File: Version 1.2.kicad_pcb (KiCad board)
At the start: 4 copper layers, 40 x 40 mm, 33 parts, among them J1 Conn_01x04_Pin, J2 Screw_Terminal_01x02, J3 Conn_01x07_Pin, J4 Conn_Coaxial, U1 BGA2801, U2 BGA420, U3 AS179-92LF, U4 SX1278, U5 74LVC1G19, Y1 ECS-TXO-2520-33-400-AN-TR

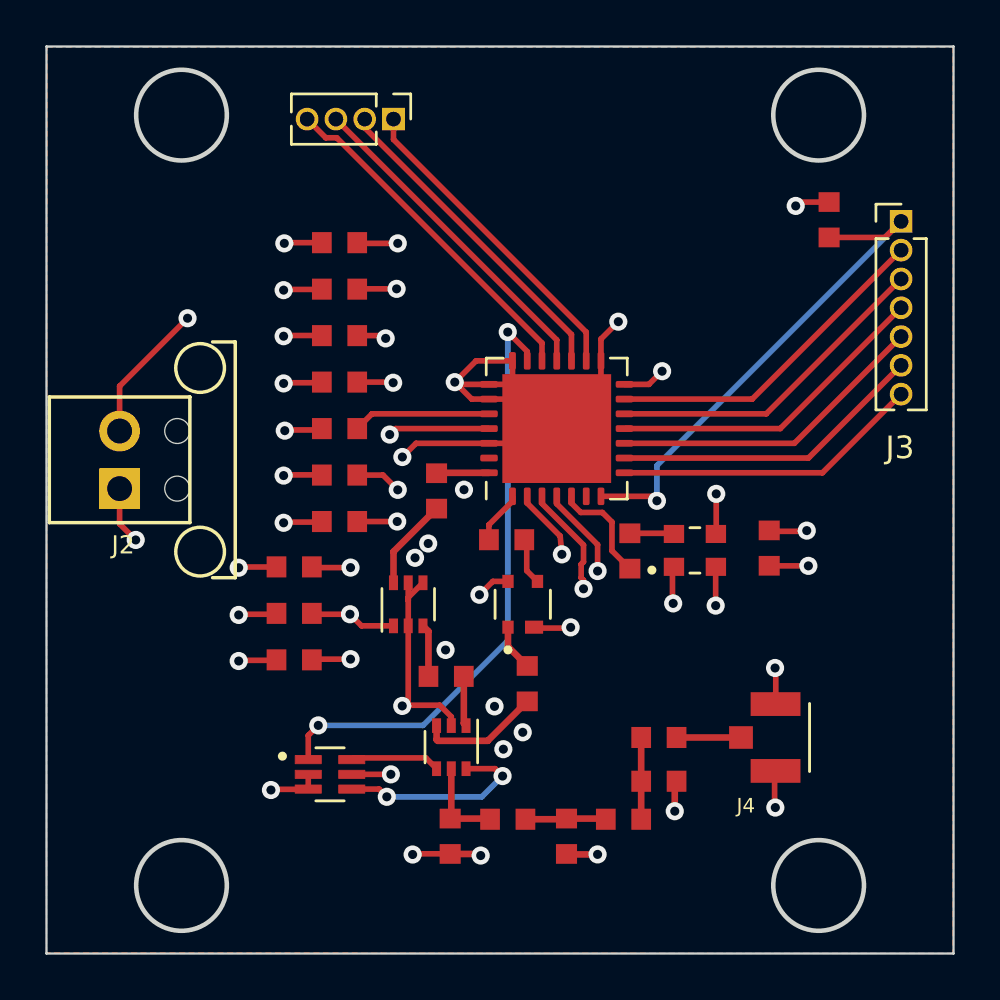
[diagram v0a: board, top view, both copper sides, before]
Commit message: EMI & Compression
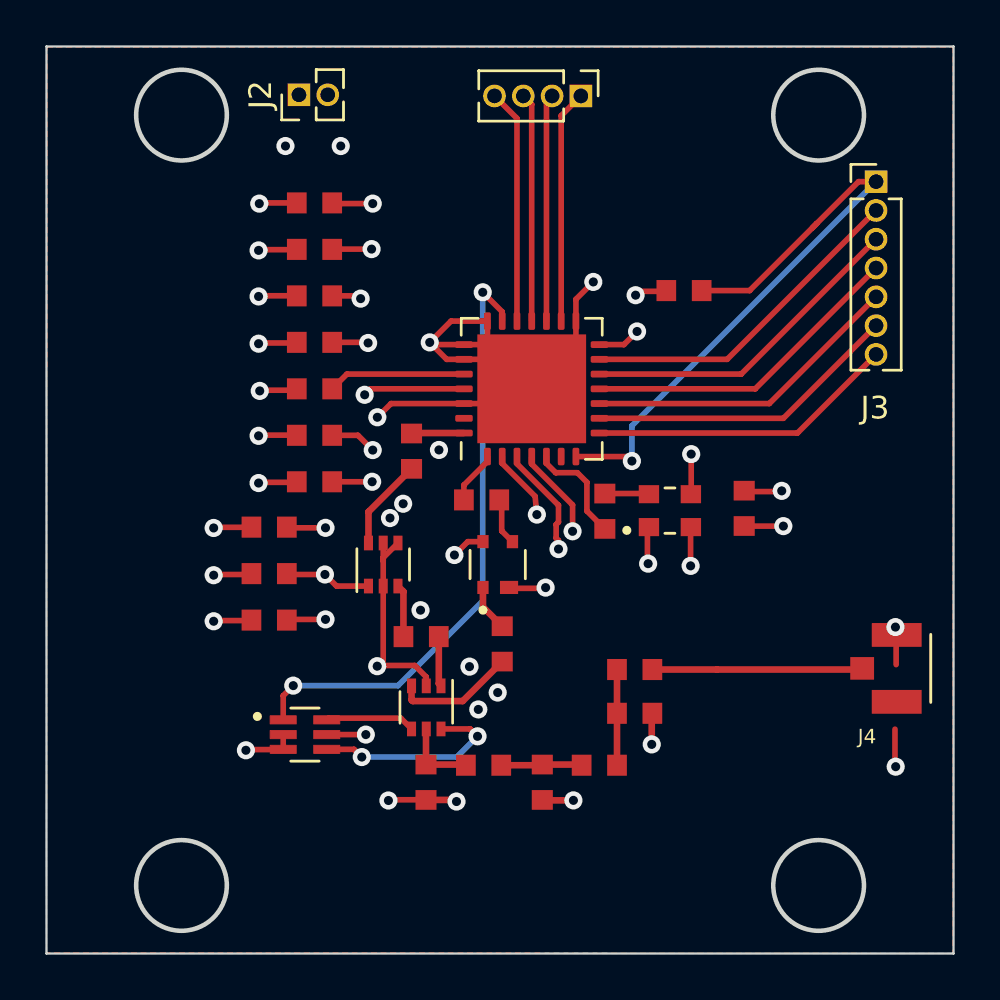
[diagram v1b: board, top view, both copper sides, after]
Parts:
- J2: value Screw_Terminal_01x02 -> Conn_01x02_Pin; footprint Screw Connector 01x02:1725656 -> Connector_PinHeader_1.27mm:PinHeader_1x02_P1.27mm_Vertical
- moved J2 16.3 mm to (127.6, 71.4)
- moved J1 8.33 mm to (140.1, 71.5)
- moved R1 7.12 mm to (144.6, 80.1), turned to 0 degrees
- moved J4 6.15 mm to (154.0, 96.7)
- moved C5 3.18 mm to (142.5, 98.7)
- moved L3 3.18 mm to (142.5, 96.8)
- moved C1 2.61 mm to (133.2, 101.7)
- moved C4 2.61 mm to (138.4, 101.7)
- moved L1 2.61 mm to (135.8, 101.0)
- moved L2 2.61 mm to (140.9, 101.0)
- moved J3 2.07 mm to (153.1, 75.3)
- moved U2 2.07 mm to (136.4, 92.1)
- moved U3 2.07 mm to (133.3, 98.4)
- moved U4 2.07 mm to (137.9, 84.4)
- moved Y1 2.07 mm to (144.0, 89.8)
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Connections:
- J2 pad 1: +3.3V -> GND
- J2 pad 2: GND -> +3.3V
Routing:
- net /Reset: track 22.8 -> 29.3 mm
- net /Filter_Output: track 2.84 -> 9.20 mm
- net /NSS: track 15.2 -> 10.3 mm
- net /MOSI: track 14.7 -> 10.1 mm
- net /MISO: track 14.4 -> 10.0 mm
- net /SCK: track 14.2 -> 10.3 mm
- net GND: track 76.6 -> 72.7 mm
- net /Filter_Input: track 3.96 -> 3.31 mm
- net Net-(C5-Pad1): track 3.61 -> 4.22 mm
